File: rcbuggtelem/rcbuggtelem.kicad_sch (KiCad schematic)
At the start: 2 parts, among them J1 Conn_01x05, J2 Conn_01x02

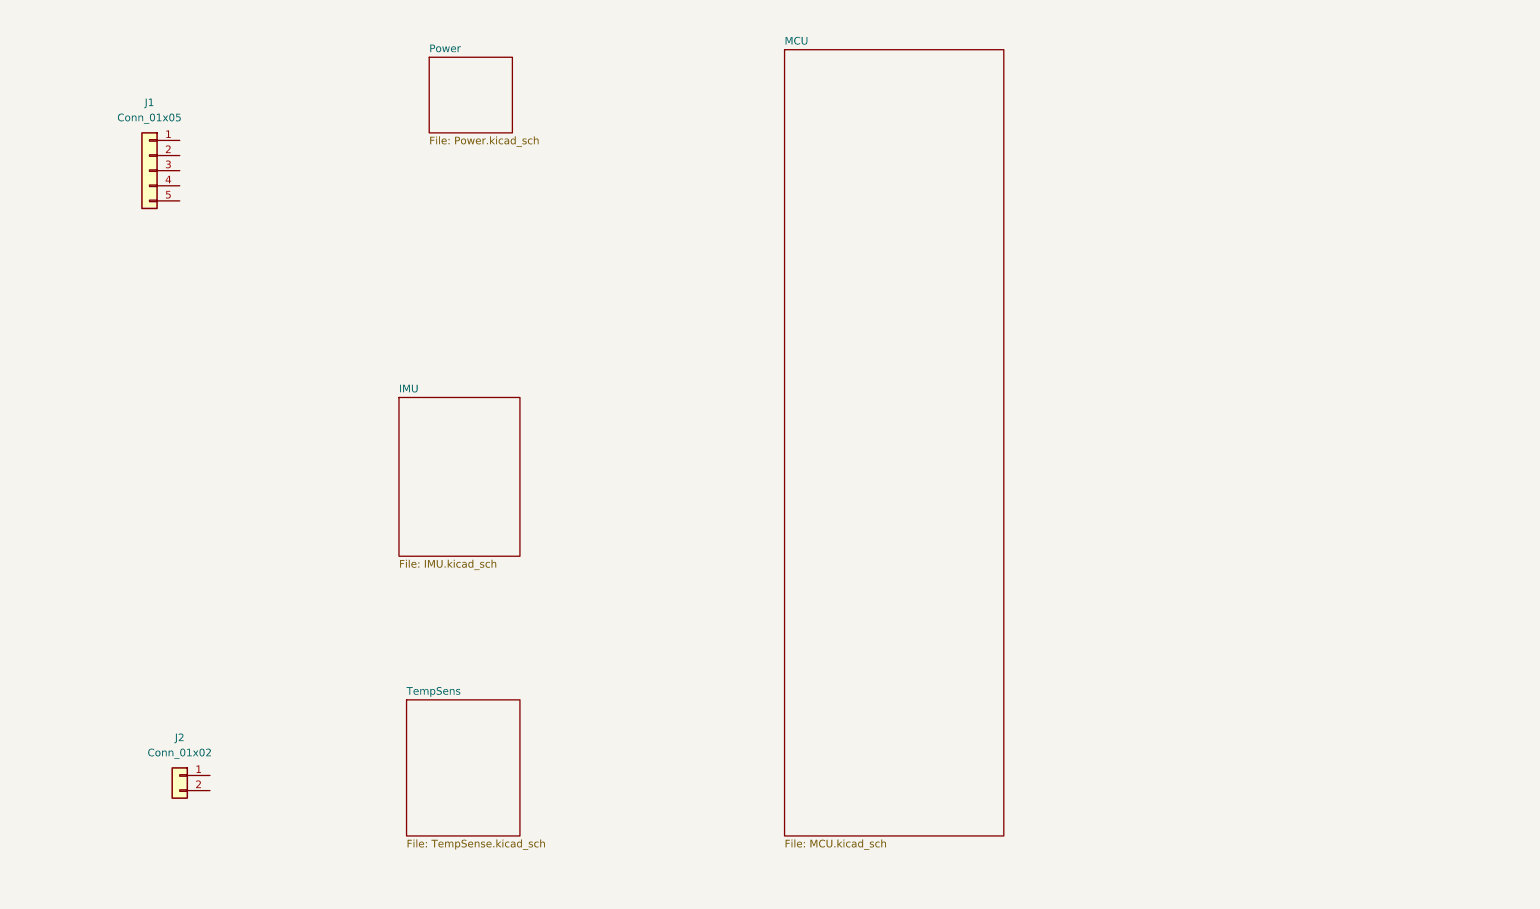
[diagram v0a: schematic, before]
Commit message: up
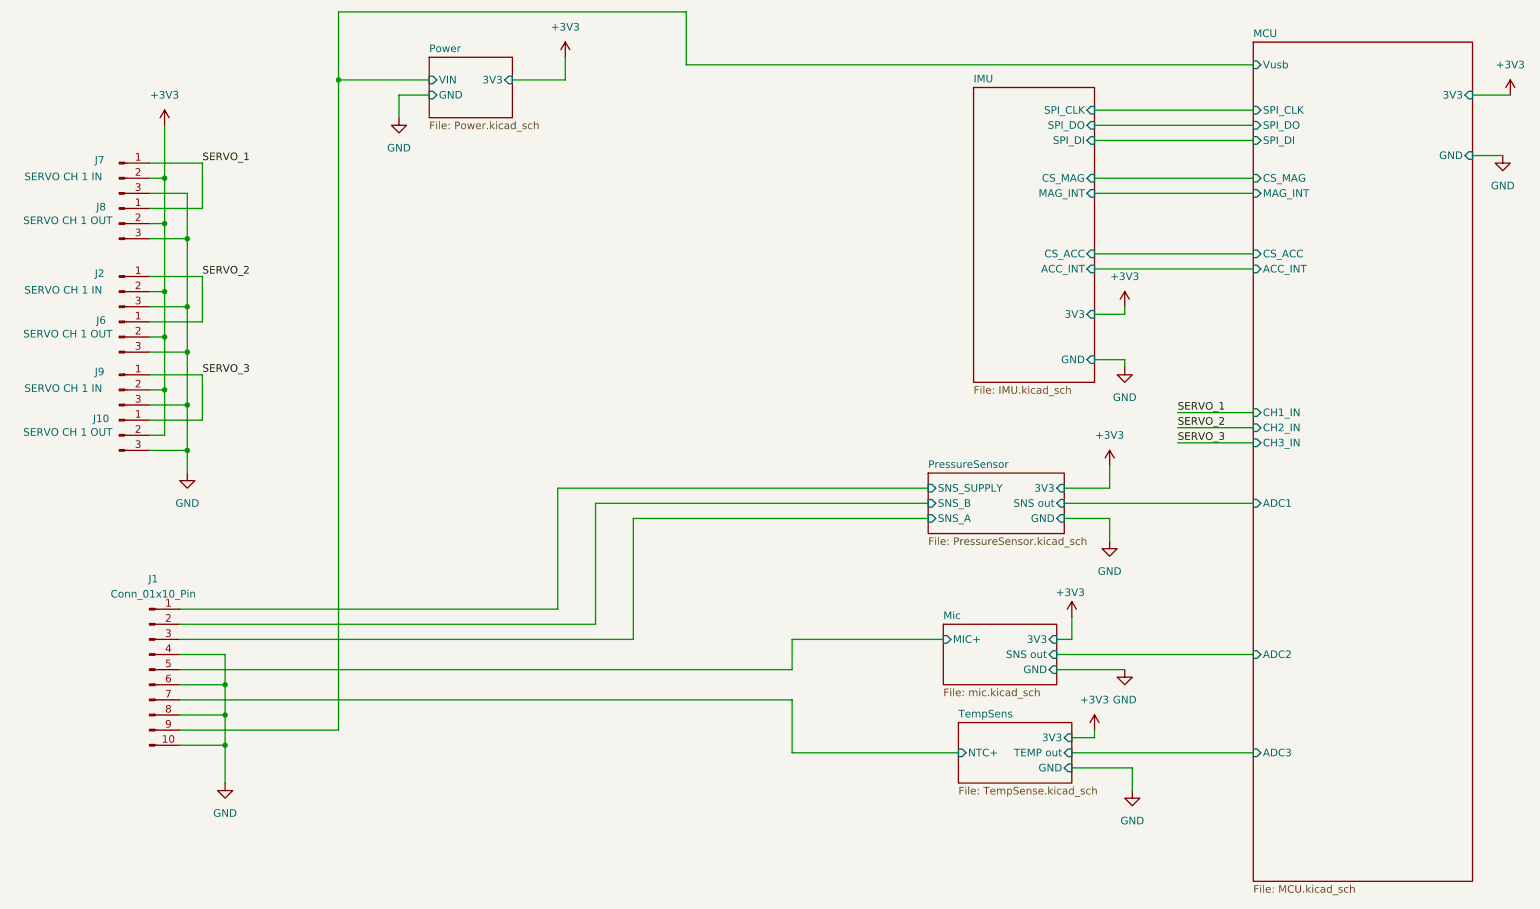
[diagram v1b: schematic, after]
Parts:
- removed J1: Conn_01x05, symbol Connector_Generic:Conn_01x05
- removed J2: Conn_01x02, symbol Connector_Generic:Conn_01x02
- added J1: Conn_01x10_Pin, Connector_PinSocket_2.54mm:PinSocket_1x10_P2.54mm_Vertical, symbol Connector:Conn_01x10_Pin
- added J10, J6, J8: SERVO CH 1 OUT, Connector_PinHeader_2.54mm:PinHeader_1x03_P2.54mm_Vertical, symbol Connector:Conn_01x03_Pin
- added J2, J7, J9: SERVO CH 1 IN, Connector_PinHeader_2.54mm:PinHeader_1x03_P2.54mm_Vertical, symbol Connector:Conn_01x03_Pin
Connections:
- new net +3V3: J10.2 (Pin_2), J2.2 (Pin_2), J6.2 (Pin_2), J7.2 (Pin_2), J8.2 (Pin_2), J9.2 (Pin_2)
- new net GND: J1.10 (Pin_10), J1.4 (Pin_4), J1.6 (Pin_6), J1.8 (Pin_8), J10.3 (Pin_3), J2.3 (Pin_3), J6.3 (Pin_3), J7.3 (Pin_3), J8.3 (Pin_3), J9.3 (Pin_3)
- new net MCU/Vusb: J1.9 (Pin_9)
- new net Mic/MIC+: J1.5 (Pin_5)
- new net PressureSensor/SNS_A: J1.3 (Pin_3)
- new net PressureSensor/SNS_B: J1.2 (Pin_2)
- new net PressureSensor/SNS_SUPPLY: J1.1 (Pin_1)
- new net SERVO_1: J7.1 (Pin_1), J8.1 (Pin_1)
- new net SERVO_2: J2.1 (Pin_1), J6.1 (Pin_1)
- new net SERVO_3: J10.1 (Pin_1), J9.1 (Pin_1)
- new net TempSens/NTC+: J1.7 (Pin_7)
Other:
- added sheet Mic (mic.kicad_sch)
- added sheet PressureSensor (PressureSensor.kicad_sch)
- sheet IMU ports: added 3V3, ACC_INT, CS_ACC, CS_MAG, GND, MAG_INT, SPI_CLK, SPI_DI, SPI_DO; removed none
- sheet MCU ports: added 3V3, ACC_INT, ADC1, ADC2, ADC3, CH1_IN, CH2_IN, CH3_IN, CS_ACC, CS_MAG, GND, MAG_INT, SPI_CLK, SPI_DI, SPI_DO, Vusb; removed none
- sheet Power ports: added 3V3, GND, VIN; removed none
- sheet TempSens ports: added 3V3, GND, NTC+, TEMP out; removed none
